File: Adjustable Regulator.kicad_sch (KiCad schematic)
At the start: 5 parts, among them U20 LM2596S-ADJ

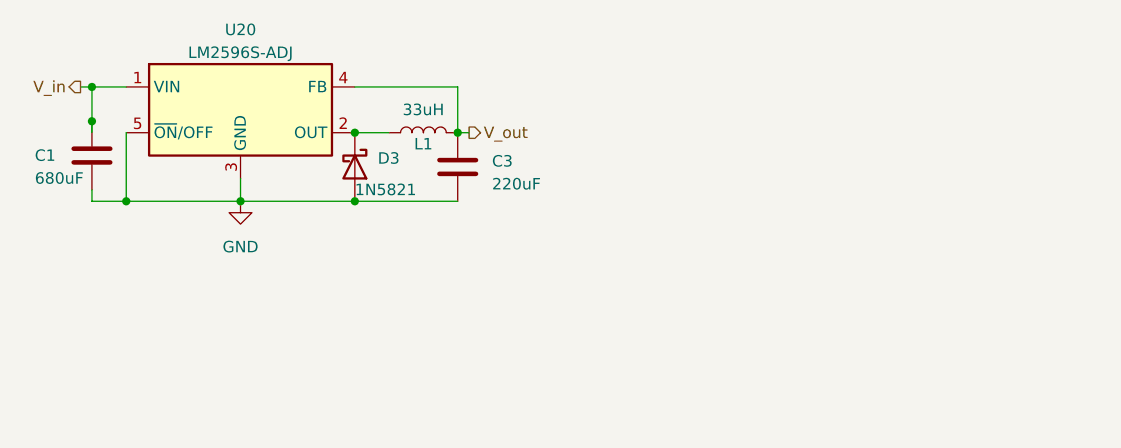
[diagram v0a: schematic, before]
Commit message: hi
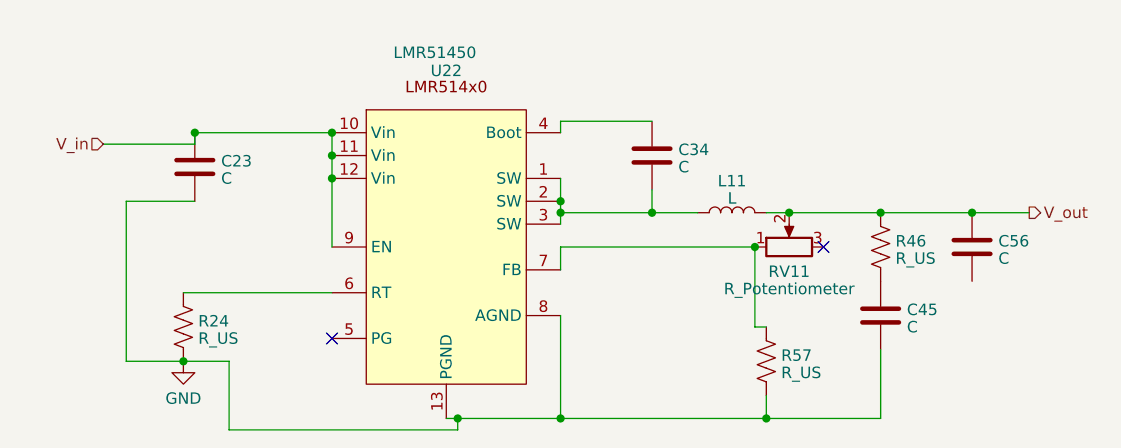
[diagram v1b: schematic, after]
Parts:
- removed C1: 680uF, symbol Device:C
- removed C3: 220uF, symbol Device:C
- removed D3: 1N5821, Diode_THT:D_DO-201AD_P15.24mm_Horizontal, symbol Diode:1N5821
- removed L1: 33uH, symbol Device:L
- removed U20: LM2596S-ADJ, Package_TO_SOT_SMD:TO-263-5_TabPin3, symbol Regulator_Switching:LM2596S-ADJ
- added C23, C34, C45, C56: C, symbol Device:C
- added L11: L, symbol Device:L
- added R24, R46, R57: R_US, symbol Device:R_US
- added RV11: R_Potentiometer, symbol Device:R_Potentiometer
- added U22: LMR51450, symbol LMR514x0:LMR514x0
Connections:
- net GND: now also C23.2, C45.2, R24.2, R57.2, U22.13 (PGND), U22.8 (AGND)
- net V_in: now also C23.1, U22.10 (Vin), U22.11 (Vin), U22.12 (Vin), U22.9 (EN)
- net V_out: now also C56.1, L11.2, R46.1, RV11.2
- new net: C34.1, U22.4 (Boot)
- new net: C34.2, L11.1, U22.1 (SW), U22.2 (SW), U22.3 (SW)
- new net: R24.1, U22.6 (RT)
- new net: R57.1, RV11.1, U22.7 (FB)
- new net: C45.1, R46.2
- no-connect marks 0 -> 2
